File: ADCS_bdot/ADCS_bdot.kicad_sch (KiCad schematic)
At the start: 0 parts

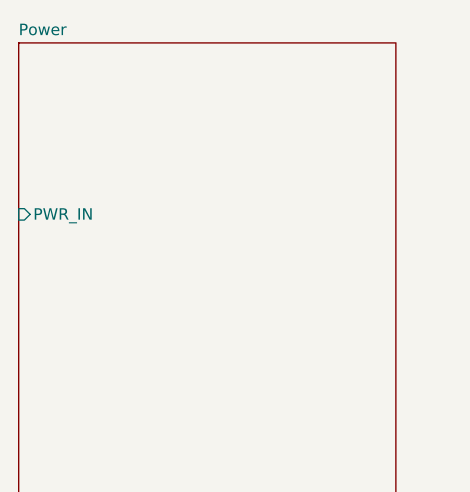
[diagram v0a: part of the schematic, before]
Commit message: add: components
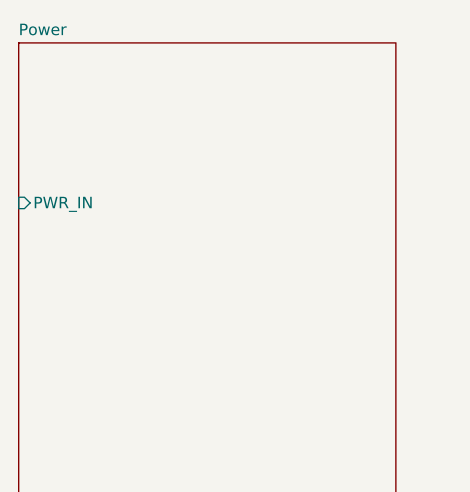
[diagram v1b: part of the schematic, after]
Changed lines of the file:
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@@
 		)
 		(pin "PWR_IN" input
-			(at 71.12 69.85 180)
+			(at 71.12 68.58 180)
 			(effects
 				(font
